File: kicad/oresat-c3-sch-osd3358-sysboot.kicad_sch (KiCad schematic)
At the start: 25 parts, among them J4 Conn_01x05, J6 Conn_01x02, U1 OSD3358-512M-BSM, U39 TCAN330

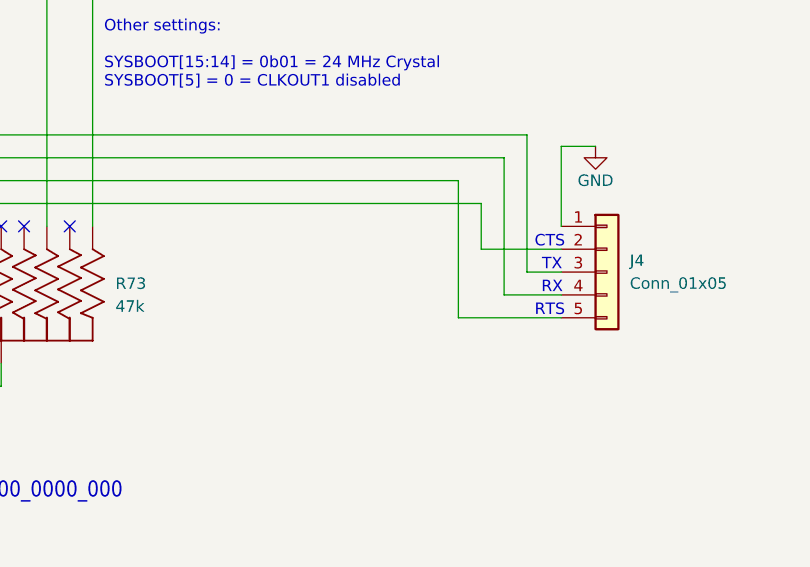
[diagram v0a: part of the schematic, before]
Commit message: - Labelled GPIOs and UART lines to processor pins - Routed UART lines - Routed GPIO Lines - Refilled zones - Added via fencing back in - Board should be ready to be reviewed now
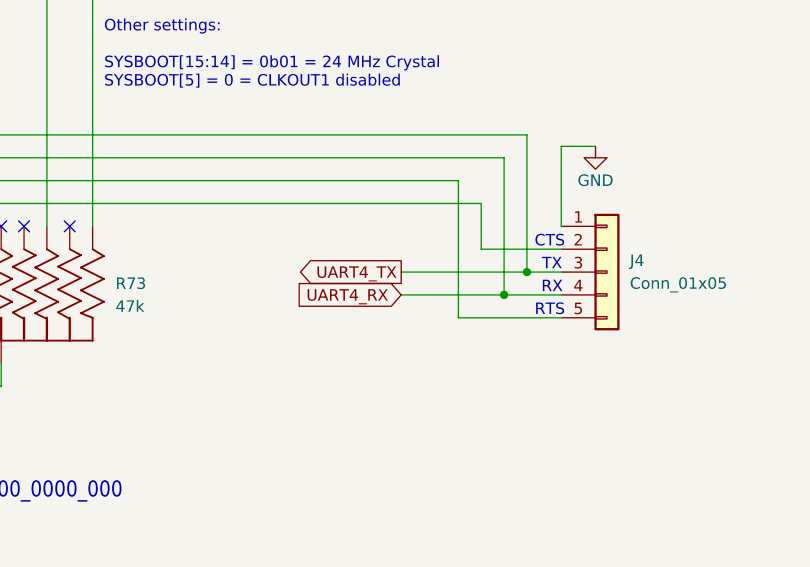
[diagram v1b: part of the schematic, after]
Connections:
- net UART4_TX: now reaches J4.3 (Pin_3), R72.4 (44), U1.J1 (LCD_DATA8)
- net UART4_RX: now reaches J4.4 (Pin_4), R72.7 (77), U1.K3 (LCD_DATA9)
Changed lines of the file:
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@@
+	)
+	(junction
+		(at 304.8 177.8)
+		(diameter 0)
+		(color 0 0 0 0)
 	)
 	(junction
@@
 	)
 	(junction
+		(at 302.26 180.34)
+		(diameter 0)
+		(color 0 0 0 0)
+	)
+	(junction
 		(at 148.59 92.71)
 		(diameter 0)
@@
 	(wire
 		(pts
+			(xy 290.83 180.34) (xy 302.26 180.34)
+		)
+		(stroke
+			(width 0)
+			(type default)
+		)
+	)
+	(wire
+		(pts
 			(xy 116.84 92.71) (xy 119.38 92.71)
 		)
@@
 		(pts
 			(xy 297.18 142.24) (xy 300.99 142.24)
+		)
+		(stroke
+			(width 0)
+			(type default)
+		)
+	)
+	(wire
+		(pts
+			(xy 290.83 177.8) (xy 304.8 177.8)
 		)
 		(stroke
@@
 		)
 	)
+	(global_label "UART4_RX"
+		(shape input)
+		(at 290.83 180.34 180)
+		(fields_autoplaced yes)
+		(effects
+			(font
+				(size 1.27 1.27)
+			)
+			(justify right)
+		)
+		(property "Intersheetrefs" "${INTERSHEET_REFS}"
+			(at 278.5315 180.34 0)
+			(effects
+				(font
+					(size 1.27 1.27)
+				)
+				(justify right)
+			)
+		)
+	)
+	(global_label "UART4_TX"
+		(shape output)
+		(at 290.83 177.8 180)
+		(fields_autoplaced yes)
+		(effects
+			(font
+				(size 1.27 1.27)
+			)
+			(justify right)
+		)
+		(property "Intersheetrefs" "${INTERSHEET_REFS}"
+			(at 278.8339 177.8 0)
+			(effects
+				(font
+					(size 1.27 1.27)
+				)
+				(justify right)
+			)
+		)
+	)

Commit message: - Configured pin headers for UART5 and boot pins to be horizontal - Removed some TPs for GPIO pins
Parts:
- J4: footprint Connector_PinHeader_2.54mm:PinHeader_1x05_P2.54mm_Vertical -> Connector_PinHeader_2.54mm:PinHeader_1x05_P2.54mm_Horizontal
- J6: footprint Connector_PinHeader_2.54mm:PinHeader_1x02_P2.54mm_Vertical -> M20-8890245:M20-8890245
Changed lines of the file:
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@@
 			)
 		)
-		(property "Footprint" "Connector_PinHeader_2.54mm:PinHeader_1x02_P2.54mm_Vertical"
+		(property "Footprint" "M20-8890245:M20-8890245"
 			(at 264.16 134.62 0)
 			(effects
@@
 			)
 		)
-		(property "Footprint" "Connector_PinHeader_2.54mm:PinHeader_1x05_P2.54mm_Vertical"
+		(property "Footprint" "Connector_PinHeader_2.54mm:PinHeader_1x05_P2.54mm_Horizontal"
 			(at 313.69 177.8 0)
 			(effects

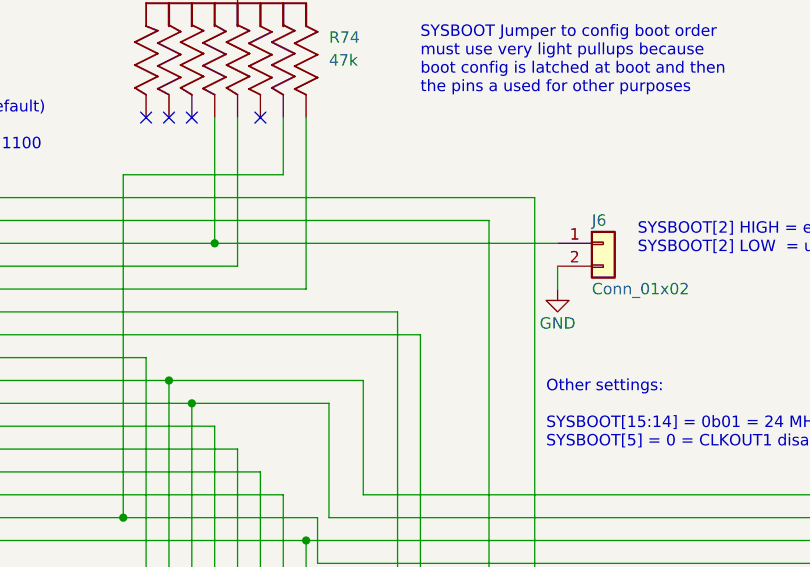
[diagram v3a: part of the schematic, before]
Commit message: - Routed New boot pin properly, added test points to old spots as backups - Filled some floating ground planes with vias near I2C2 Buffer - Routed UART0 to new pins properly - Fixed SD card connector, it somehow got moved - Fixed som DRC issues, still need to go through a lot - Labelled CSKB, added x to anything unconnected
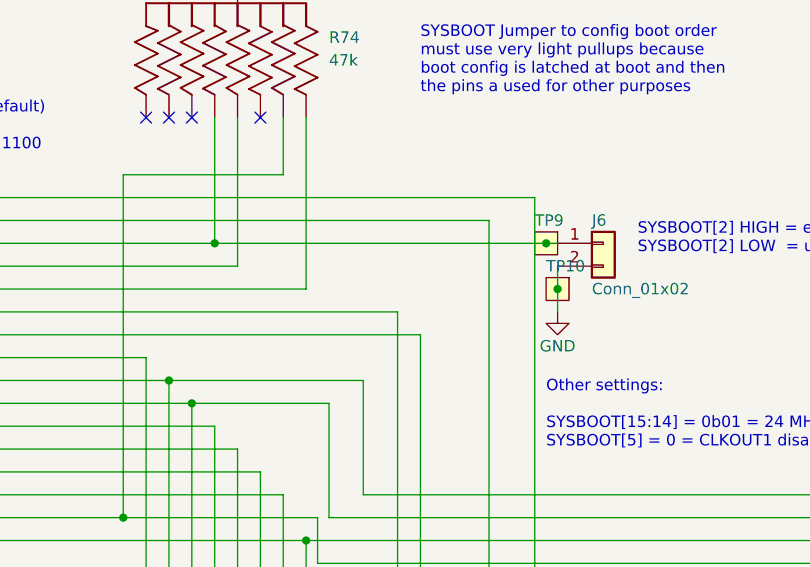
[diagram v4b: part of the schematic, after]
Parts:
- added TP10, TP9: Test-Point, oresat-misc:TestPoint-0.75mm-th, symbol oresat-misc:Test-Point-0.75mm-th
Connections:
- net GND: now also TP10.1
- net at J6.1 (Pin_1), R74.8 (88), U1.G1 (LCD_DATA2): now also TP9.1
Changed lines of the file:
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@@
 	)
 	(junction
+		(at 259.08 139.7)
+		(diameter 0)
+		(color 0 0 0 0)
+	)
+	(junction
+		(at 257.81 134.62)
+		(diameter 0)
+		(color 0 0 0 0)
+	)
+	(junction
 		(at 302.26 180.34)
 		(diameter 0)
@@
 	(wire
 		(pts
-			(xy 220.98 134.62) (xy 259.08 134.62)
+			(xy 220.98 134.62) (xy 257.81 134.62)
 		)
 		(stroke
@@
 	(wire
 		(pts
+			(xy 259.08 139.7) (xy 259.08 142.24)
+		)
+		(stroke
+			(width 0)
+			(type default)
+		)
+	)
+	(wire
+		(pts
 			(xy 107.95 177.8) (xy 116.84 177.8)
 		)
@@
 	(wire
 		(pts
+			(xy 257.81 134.62) (xy 259.08 134.62)
+		)
+		(stroke
+			(width 0)
+			(type default)
+		)
+	)
+	(wire
+		(pts
 			(xy 107.95 157.48) (xy 116.84 157.48)
 		)
@@
 	)
 	(symbol
+		(lib_id "oresat-misc:Test-Point-0.75mm-th")
+		(at 259.08 139.7 270)
+		(unit 1)
+		(exclude_from_sim no)
+		(in_bom yes)
+		(on_board yes)
+		(dnp no)
+		(property "Reference" "TP10"
+			(at 257.81 137.16 90)
+			(effects
+				(font
+					(size 1.27 1.27)
+				)
+				(justify left)
+			)
+		)
+		(property "Value" "Test-Point"
+			(at 261.62 139.7 0)
+			(effects
+				(font
+					(size 1.27 1.27)
+				)
+				(hide yes)
+			)
+		)
+		(property "Footprint" "oresat-misc:TestPoint-0.75mm-th"
+			(at 269.24 139.7 0)
+			(effects
+				(font
+					(size 1.27 1.27)
+				)
+				(hide yes)
+			)
+		)
+		(property "Datasheet" ""
+			(at 259.08 139.7 0)
+			(effects
+				(font
+					(size 1.27 1.27)
+				)
+				(hide yes)
+			)
+		)
+		(property "Description" ""
+			(at 259.08 139.7 0)
+			(effects
+				(font
+					(size 1.27 1.27)
+				)
+				(hide yes)
+			)
+		)
+		(property "Part Page" ""
+			(at 259.08 139.7 0)
+			(effects
+				(font
+					(size 1.27 1.27)
+				)
+				(hide yes)
+			)
+		)
+		(property "Price" ""
+			(at 259.08 139.7 0)
+			(effects
+				(font
+					(size 1.27 1.27)
+				)
+				(hide yes)
+			)
+		)
+		(property "Total Price" ""
+			(at 259.08 139.7 0)
+			(effects
+				(font
+					(size 1.27 1.27)
+				)
+				(hide yes)
+			)
+		)
+		(pin "1"
+		)
+		(instances
+			(project "oresat-c3"
+				(path "/65d12cdd-c326-4033-9053-c59fa4e0b25e/0c732c1e-ab0d-41ac-9d77-9d7763333b6f"
+					(reference "TP10")
+					(unit 1)
+				)
+			)
+		)
+	)
+	(symbol
 		(lib_id "Connector_Generic:Conn_01x02")
 		(at 264.16 134.62 0)
@@
 	(symbol
 		(lib_id "power:GND")
-		(at 259.08 139.7 0)
+		(at 259.08 142.24 0)
 		(unit 1)
 		(exclude_from_sim no)
@@
 		(dnp no)
 		(property "Reference" "#PWR0160"
-			(at 259.08 146.05 0)
+			(at 259.08 148.59 0)
 			(effects
 				(font
@@
 		)
 		(property "Value" "GND"
-			(at 259.08 143.51 0)
+			(at 259.08 146.05 0)
 			(effects
 				(font
@@
 		)
 		(property "Footprint" ""
-			(at 259.08 139.7 0)
+			(at 259.08 142.24 0)
 			(effects
 				(font
@@
 		)
 		(property "Datasheet" ""
-			(at 259.08 139.7 0)
+			(at 259.08 142.24 0)
 			(effects
 				(font
@@
 		)
 		(property "Description" ""
-			(at 259.08 139.7 0)
+			(at 259.08 142.24 0)
 			(effects
 				(font
@@
 					(unit 1)
 				)
+			)
+		)
+	)
+	(symbol
+		(lib_id "oresat-misc:Test-Point-0.75mm-th")
+		(at 257.81 134.62 270)
+		(unit 1)
+		(exclude_from_sim no)
+		(in_bom yes)
+		(on_board yes)
+		(dnp no)
+		(property "Reference" "TP9"
+			(at 256.54 132.08 90)
+			(effects
+				(font
+					(size 1.27 1.27)
+				)
+				(justify left)
+			)
+		)
+		(property "Value" "Test-Point"
+			(at 260.35 134.62 0)
+			(effects
+				(font
+					(size 1.27 1.27)
+				)
+				(hide yes)
+			)
+		)
+		(property "Footprint" "oresat-misc:TestPoint-0.75mm-th"
+			(at 267.97 134.62 0)
+			(effects
+				(font
+					(size 1.27 1.27)
+				)
+				(hide yes)
+			)
+		)
+		(property "Datasheet" ""
+			(at 257.81 134.62 0)
+			(effects
+				(font
+					(size 1.27 1.27)
+				)
+				(hide yes)
+			)
+		)
+		(property "Description" ""
+			(at 257.81 134.62 0)
+			(effects
+				(font
+					(size 1.27 1.27)
+				)
+				(hide yes)
+			)
+		)
+		(property "Part Page" ""
+			(at 257.81 134.62 0)
+			(effects
+				(font
+					(size 1.27 1.27)
+				)
+				(hide yes)
+			)
+		)
+		(property "Price" ""
+			(at 257.81 134.62 0)
+			(effects
+				(font
+					(size 1.27 1.27)
+				)
+				(hide yes)
+			)
+		)
+		(property "Total Price" ""
+			(at 257.81 134.62 0)
+			(effects
+				(font
+					(size 1.27 1.27)
+				)
+				(hide yes)
+			)
+		)
+		(pin "1"
+		)
+		(instances
+			(project "oresat-c3"
+				(path "/65d12cdd-c326-4033-9053-c59fa4e0b25e/0c732c1e-ab0d-41ac-9d77-9d7763333b6f"
+					(reference "TP9")
+					(unit 1)
+				)
